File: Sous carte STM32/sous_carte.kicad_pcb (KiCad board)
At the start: 2 copper layers, 95 x 120 mm, 35 parts, among them J1 RJ45, P1 CONN_25X2, P2 CONN_25X2, P3 CONN_10, P4 CONN_10, P5 CONN_25X2, P6 CONN_2, P7 CONN_2, P8 CONN_2

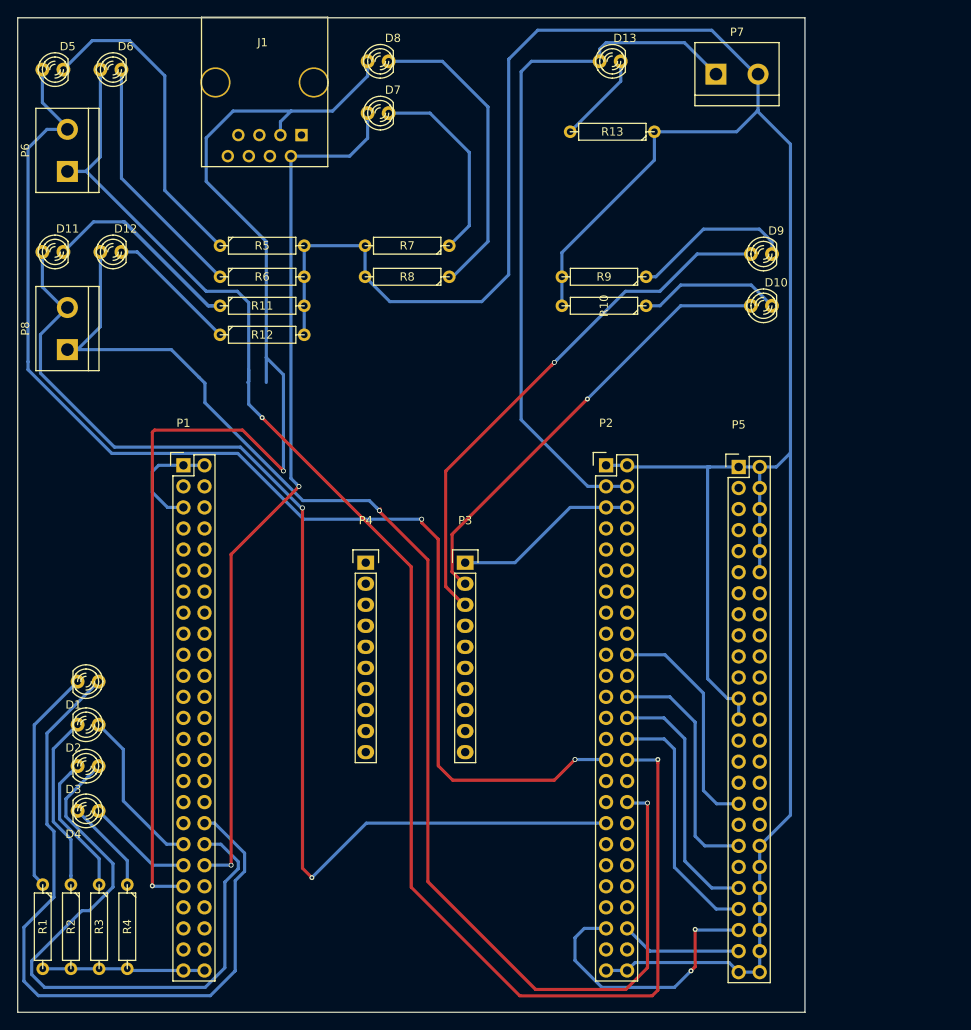
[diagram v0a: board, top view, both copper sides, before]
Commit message: essayé d'avancer
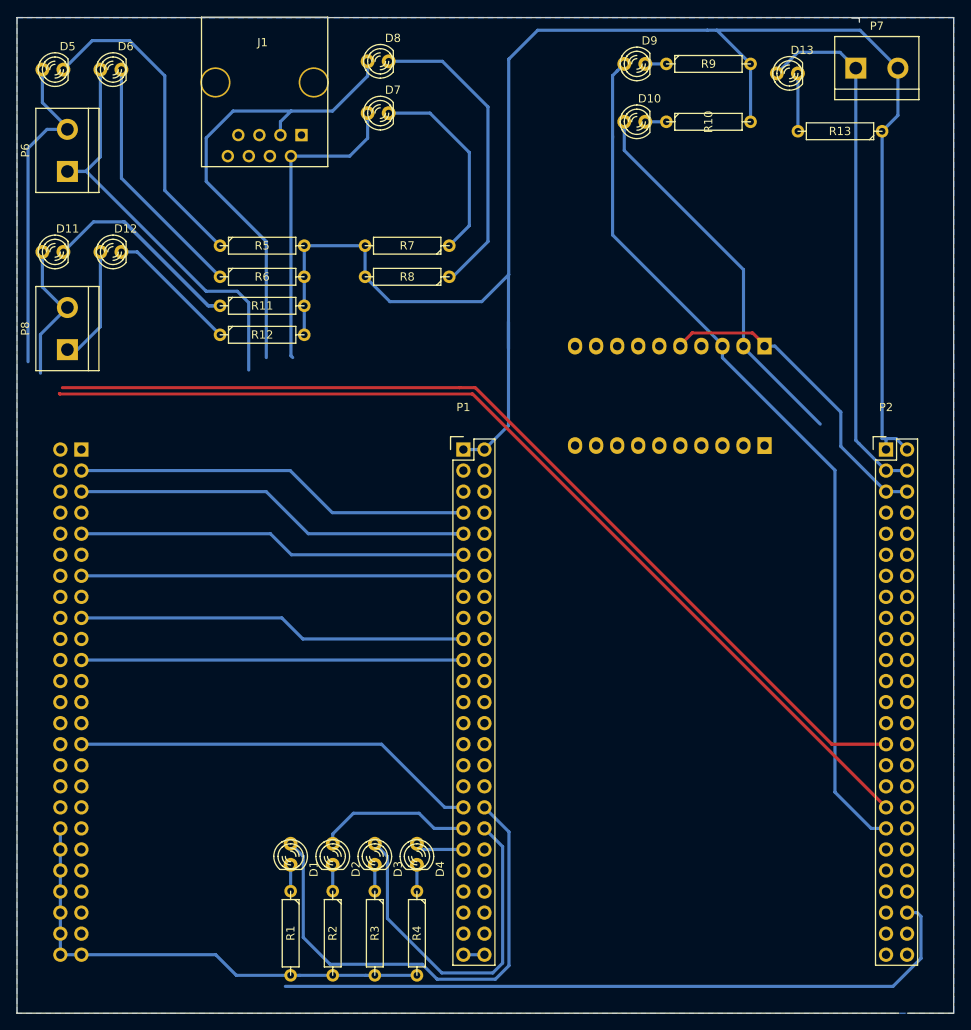
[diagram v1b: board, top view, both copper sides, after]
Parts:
- P3, P4, P5: moved to B.Cu
- moved P5 79.3 mm to (97.7, 98.1), turned to 180 degrees
- moved P4 50.2 mm to (180.1, 97.6), turned to 90 degrees
- moved P3 44.6 mm to (180.1, 85.6), turned to 90 degrees
- moved D4 40.0 mm to (138.2, 146.9), turned to 270 degrees
- moved D3 36.2 mm to (133.1, 146.9), turned to 270 degrees
- moved R4 35.0 mm to (138.2, 156.5)
- moved P1 33.8 mm to (143.8, 98.1)
- moved P2 33.8 mm to (194.8, 98.1)
- moved D2 33.4 mm to (128.0, 146.9), turned to 270 degrees
- moved R3 33.3 mm to (133.1, 156.5)
- moved D1 32.1 mm to (122.9, 146.9), turned to 270 degrees
- moved R2 31.6 mm to (128.0, 156.5)
- moved R1 29.9 mm to (122.9, 156.5)
- moved R9 28.6 mm to (173.4, 51.6), turned to 0 degrees
- moved D9 27.6 mm to (164.5, 51.6)
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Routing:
- net UART5_RX: track 163.9 -> 12.9 mm, vias 2 -> 0
- net D6: track 190.9 -> 51.8 mm, vias 2 -> 0
- net GND: track 373.7 -> 271.1 mm
- net D9: track 151.3 -> 57.3 mm, vias 2 -> 0
- net C9: track 14.6 -> 85.0 mm
- net D8: track 105.7 -> 37.6 mm, vias 2 -> 0
- net C1: track 0.00 -> 49.4 mm
- net C3: track 0.00 -> 49.4 mm
- net B11: track 0.00 -> 49.2 mm
- net C5: track 0.00 -> 47.1 mm
- net A1: track 0.00 -> 47.1 mm
- net B1: track 0.00 -> 46.1 mm
- net A3: track 0.00 -> 46.1 mm
- net UART4_TX: track 64.9 -> 107.8 mm, vias 1 -> 0
- net C8: track 33.6 -> 0.00 mm, vias 2 -> 0
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- added copper zone on B.Cu, net GND
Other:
- board size 95 x 120 mm -> 113 x 120.1 mm
